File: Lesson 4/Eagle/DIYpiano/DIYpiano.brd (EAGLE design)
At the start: 115.6 x 57.1 mm, 21 parts, among them IC1 NE555N, SW1 MOMENTARY-SWITCH-SPST-PTH-6.0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, SW2 MOMENTARY-SWITCH-SPST-PTH-6.0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, SW3 MOMENTARY-SWITCH-SPST-PTH-6.0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, SW4 MOMENTARY-SWITCH-SPST-PTH-6.0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, SW5 MOMENTARY-SWITCH-SPST-PTH-6.0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, SW6 MOMENTARY-SWITCH-SPST-PTH-6.0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, SW7 MOMENTARY-SWITCH-SPST-PTH-6.0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, SW8 MOMENTARY-SWITCH-SPST-PTH-6.0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

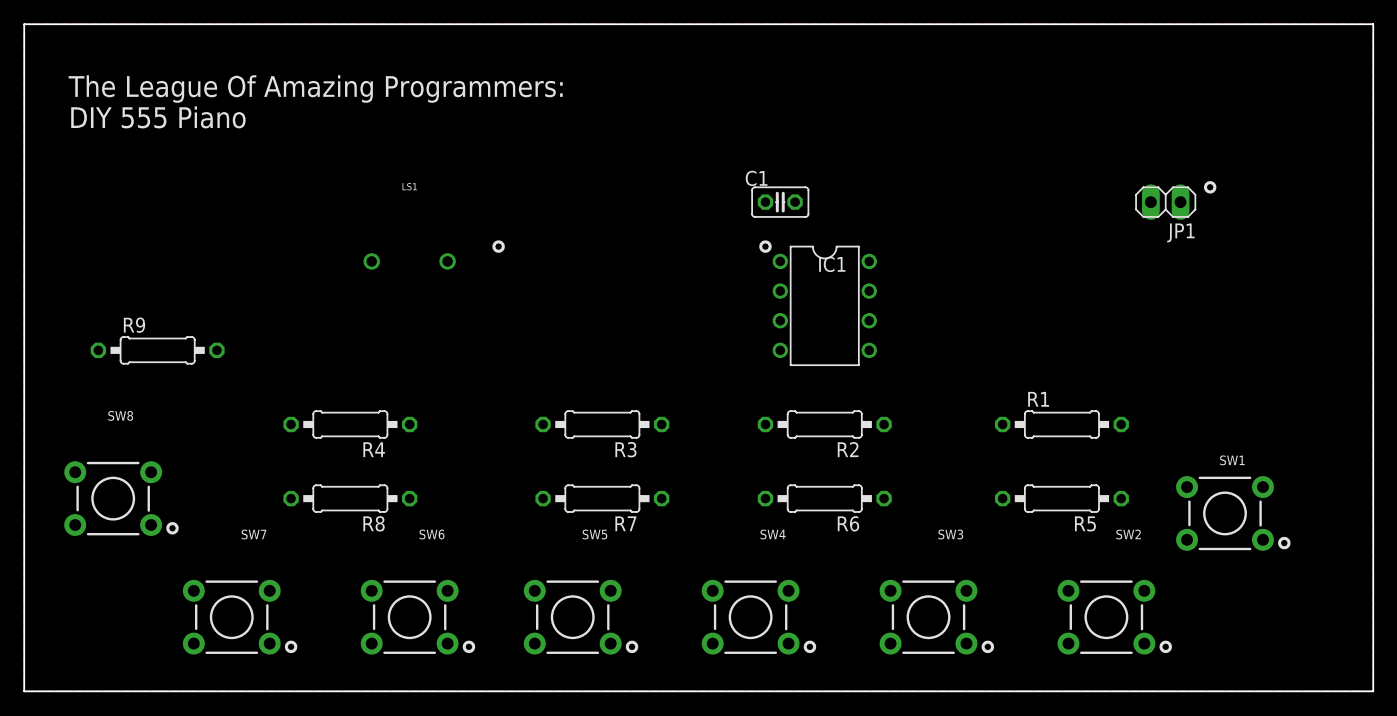
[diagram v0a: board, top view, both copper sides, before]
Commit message: Completed SCH
.
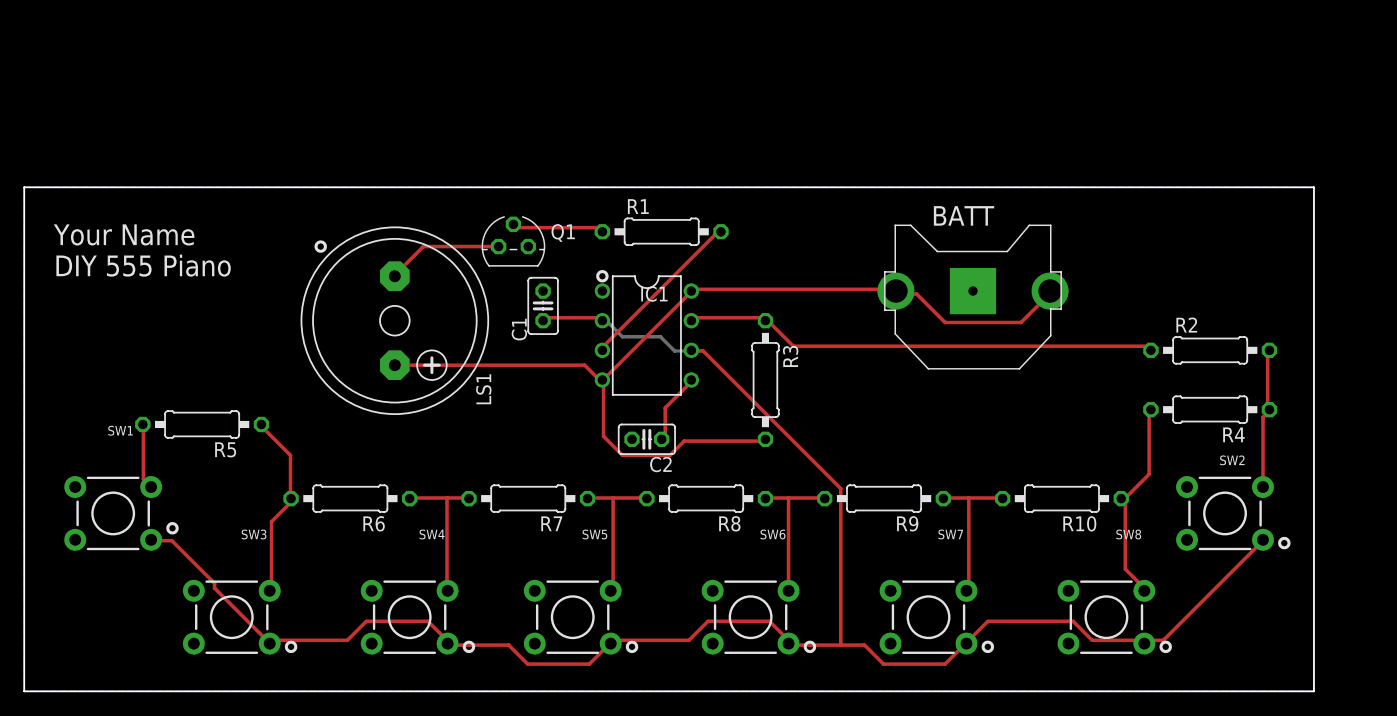
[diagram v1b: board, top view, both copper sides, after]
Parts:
- removed JP1: (no value), pinhead:1X02
- added BATT: 3V, adafruit:CR1220-THM
- added C2: 100nF, rcl:C025-025X050
- added Q1: 2N2222, transistor:TO92-E1
- added R10: 910, rcl:0207/10
- C1: value 100n -> 100nF
- LS1: value BUZZER-PTH_NO_SILK -> AT-1220-TT-3V-2-R; device SparkFun-Electromechanical:BUZZER-12MM-NS -> buzzer:F/HMB
- R3: value 390 -> 1K
- R4: value 910 -> 390
- R5: value 1K -> 1.5K
- R6: value 1.1K -> 1.3K
- R8: value 1.3K -> 1.1K
- R9: value 1.5K -> 1K
- moved SW1 95.2 mm to (6.35, 17.8)
- moved SW8 85.7 mm to (91.4, 8.89)
- moved R5 73.9 mm to (14.0, 25.4)
- moved R4 73.7 mm to (100.3, 26.7)
- moved R9 63.5 mm to (72.4, 19.1), turned to 180 degrees
- moved SW3 59.7 mm to (16.5, 8.89)
- moved SW7 59.7 mm to (76.2, 8.89)
- moved R6 40.6 mm to (26.7, 19.1)
- moved R1 38.1 mm to (53.3, 41.9)
- moved R2 33.6 mm to (100.3, 31.8), turned to 0 degrees
- moved R8 30.5 mm to (57.1, 19.1)
- moved SW4 29.2 mm to (31.8, 8.89)
- moved SW6 29.2 mm to (61.0, 8.89)
- moved C1 22.2 mm to (43.2, 35.6), turned to 90 degrees
- moved IC1 15.5 mm to (52.1, 33.0)
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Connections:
- new net N$12: C2.1, IC1.5
- new net N$13: LS1.-, Q1.1
- new net N$14: Q1.2, R1.1
- net GND: now also BATT.-, C2.2, Q1.3; no longer JP1.1, LS1.-
- net N$1: now also R4.1, SW2.3; no longer R3.1, SW1.3
- net N$10: now also R5.2, SW1.3; no longer R9.2, SW8.3
- net N$11: now also R1.2; no longer LS1.+
- net N$2: now also R3.1; no longer R1.1
- net N$4: now also R10.1, R4.2, SW8.3; no longer R3.2, R4.1, SW2.3
- net N$5: now also R10.2, R9.1, SW7.3; no longer R4.2, R5.1, SW3.3
- net N$6: now also R8.1, R9.2, SW6.3; no longer R5.2, R6.1, SW4.3
- net N$7: now also R8.2; no longer R6.2
- net N$8: now also R6.1, SW4.3; no longer R8.1, SW6.3
- net N$9: now also R5.1, R6.2, SW3.3; no longer R8.2, R9.1, SW7.3
- net VCC: now also BATT.+1, BATT.+2, LS1.+, R3.2; no longer JP1.2, R1.2
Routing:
- net N$3: track 0.00 -> 156.3 mm
- net VCC: track 0.00 -> 82.3 mm
- net N$2: track 0.00 -> 40.8 mm
- net N$4: track 0.00 -> 17.5 mm
- net N$9: track 0.00 -> 16.0 mm
- net N$11: track 0.00 -> 14.5 mm
- net N$5: track 0.00 -> 13.1 mm
- net N$7: track 0.00 -> 13.1 mm
- net N$8: track 0.00 -> 13.0 mm
- net N$6: track 0.00 -> 13.0 mm
- net N$1: track 0.00 -> 12.1 mm
- net N$13: track 0.00 -> 10.0 mm
- net N$14: track 0.00 -> 8.06 mm
- net N$12: track 0.00 -> 6.12 mm
- net N$10: track 0.00 -> 5.63 mm
- added copper zone on layer 16, net GND
- removed copper zone on layer 1, net GND
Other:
- board size 115.6 x 57.1 mm -> 110.5 x 43.2 mm
- board text added: "Your Name DIY 555 Piano"
- board text removed: "The League Of Amazing Programmers: DIY 555 Piano"
